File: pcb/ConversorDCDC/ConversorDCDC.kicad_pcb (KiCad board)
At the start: 2 copper layers, 29 x 23 mm, 28 parts, among them CN1 USBA_FEMALE, T1 MMUN2133LT1G, U1 TPS61090, X2 3.5mm

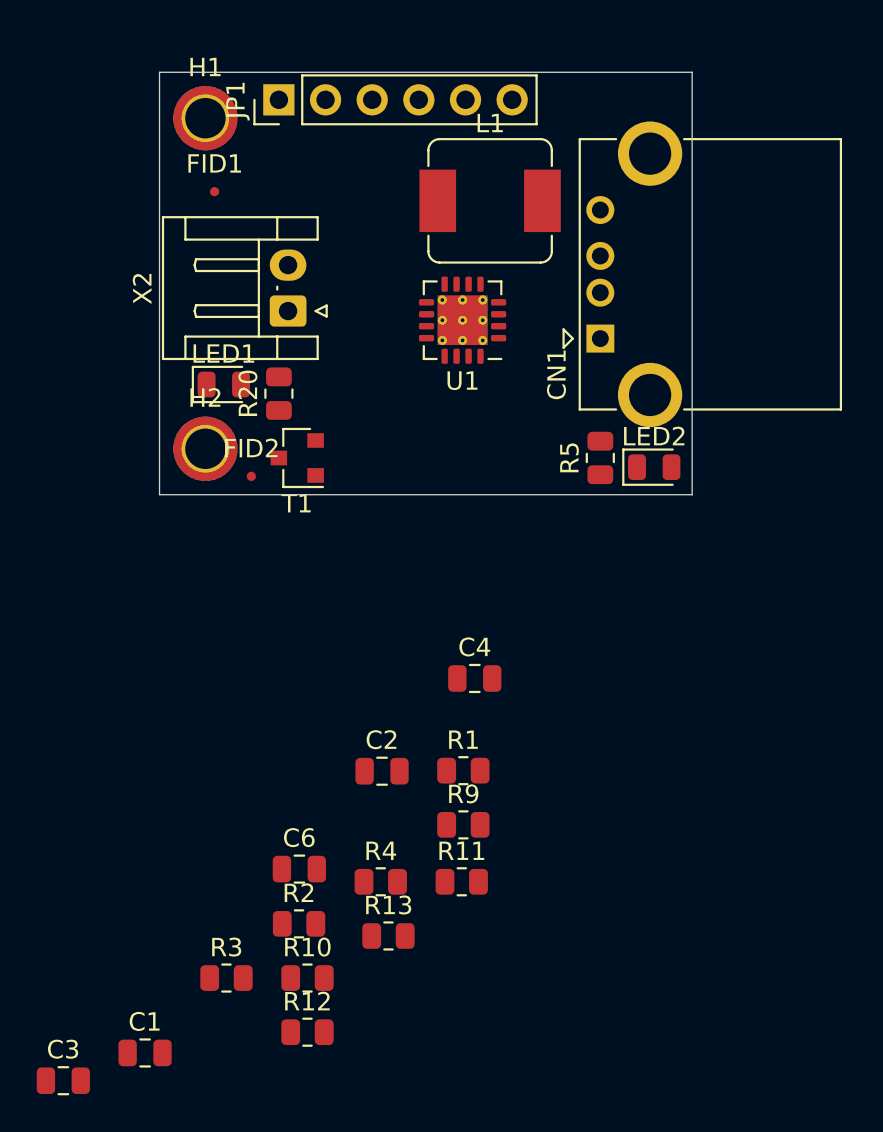
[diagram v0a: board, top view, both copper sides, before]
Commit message: ruteo de pcb
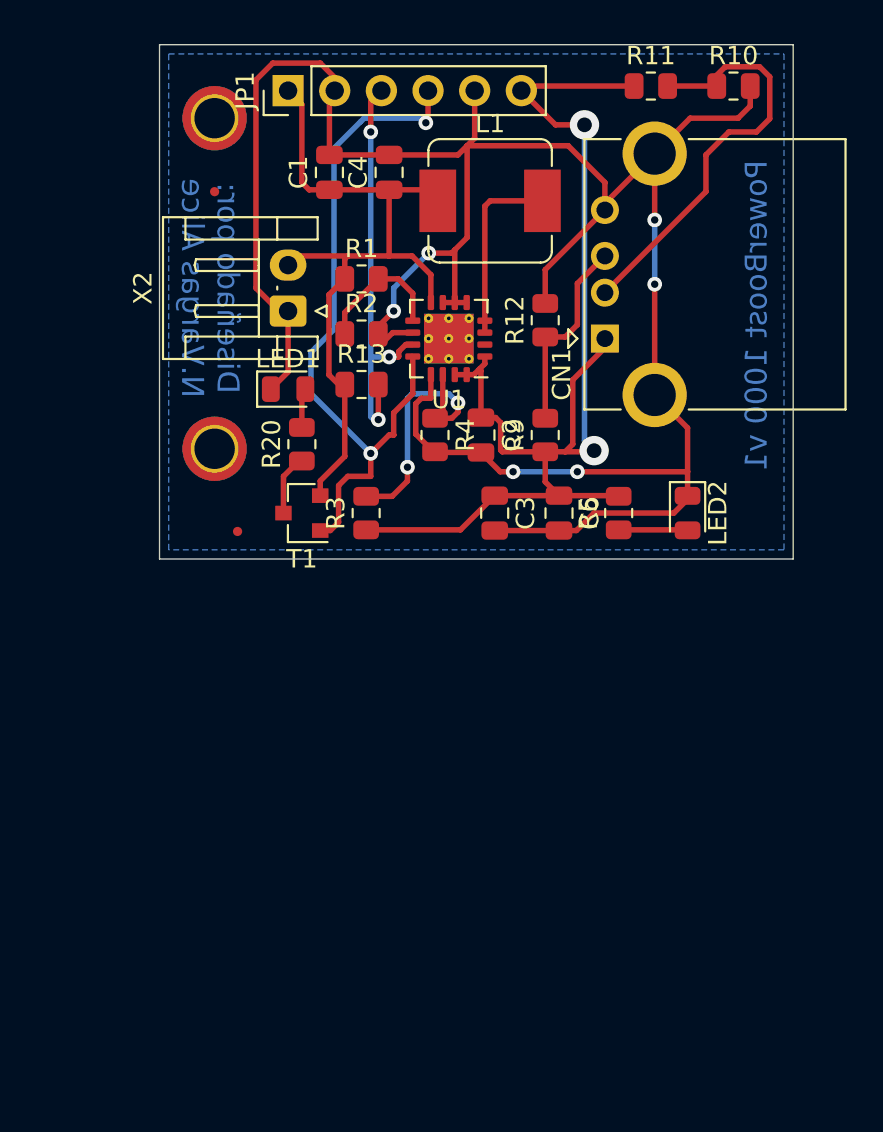
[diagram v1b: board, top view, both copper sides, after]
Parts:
- moved R10 53.8 mm to (111.2, 100.8)
- moved C1 49.0 mm to (89.2, 105.5), turned to 90 degrees
- moved R11 44.5 mm to (106.8, 100.8)
- moved R12 40.9 mm to (101.0, 113.5), turned to 90 degrees
- moved C3 38.8 mm to (98.2, 124.0), turned to 270 degrees
- moved R2 32.3 mm to (91.0, 114.2)
- moved R13 30.1 mm to (91.0, 117.0)
- moved C4 27.9 mm to (92.5, 105.5), turned to 90 degrees
- moved R1 27.3 mm to (91.0, 111.2)
- moved R3 26.4 mm to (91.2, 124.0), turned to 90 degrees
- moved R4 24.5 mm to (95.0, 119.8), turned to 270 degrees
- moved C6 24.0 mm to (101.8, 124.0), turned to 270 degrees
- moved R9 21.7 mm to (101.0, 119.8), turned to 90 degrees
- moved C2 19.1 mm to (97.5, 119.8), turned to 270 degrees
- moved LED1 3.51 mm to (87.0, 117.2)
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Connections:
- R13 pad 2: +BATT -> /ENABLE
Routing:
- net GND: track 0.00 -> 135.4 mm, vias 0 -> 6
- net +5V: track 0.00 -> 65.5 mm, vias 0 -> 2
- net +BATT: track 0.00 -> 41.6 mm
- net /LBO: track 0.00 -> 38.9 mm, vias 0 -> 2
- net /ENABLE: track 0.00 -> 23.4 mm, vias 0 -> 3
- net Net-(CN1-Pad2): track 0.00 -> 22.9 mm
- net Net-(R3-Pad2): track 0.00 -> 14.6 mm, vias 0 -> 2
- net Net-(CN1-Pad3): track 0.00 -> 10.8 mm
- net Net-(L1-Pad2): track 0.00 -> 10.1 mm
- net Net-(R1-Pad2): track 0.00 -> 7.44 mm
- net Net-(LED2-Pad2): track 0.00 -> 3.76 mm
- net Net-(R20-Pad1): track 0.00 -> 3.35 mm
- net Net-(LED1-Pad2): track 0.00 -> 2.17 mm
- added copper zone on B.Cu, net GND
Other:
- board size 29 x 23 mm -> 34.5 x 28 mm
- net class Default: clearance 0.5 -> 0.2
- rule trace_clearance: 0.5 -> 0.2
- board text added: "Diseñado por: N.Vargas Alice"
- board text added: "Mínimos (fabricante): 10 mils Grillas: 1mm, 0.5 mm, 0.25 mm Vias: 0.8/0.4 mm Margen: 0.5 mm Pista: 0.3 mm Dist. a borde: 0.5 mm Terminación: a determinar"
- board text added: "PowerBoost 1000 v1"
